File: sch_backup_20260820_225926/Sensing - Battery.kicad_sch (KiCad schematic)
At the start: 3 parts

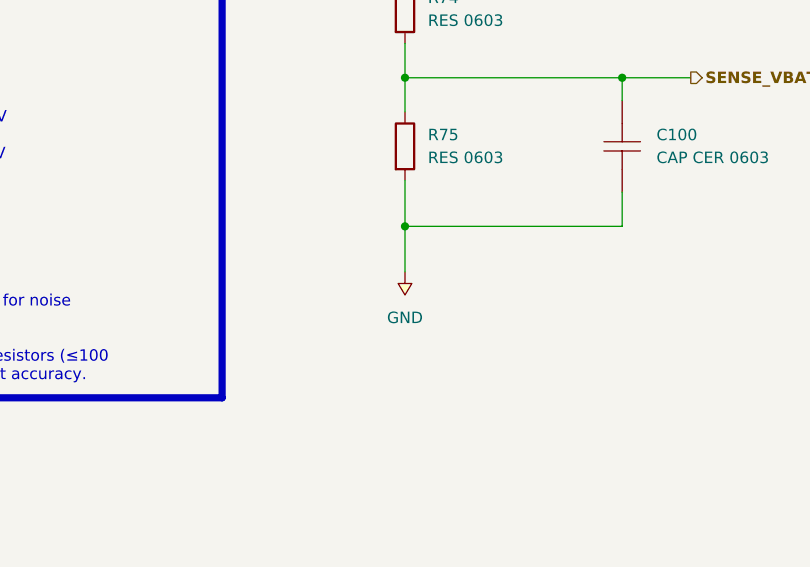
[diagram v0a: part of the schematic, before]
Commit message: Update Schematic
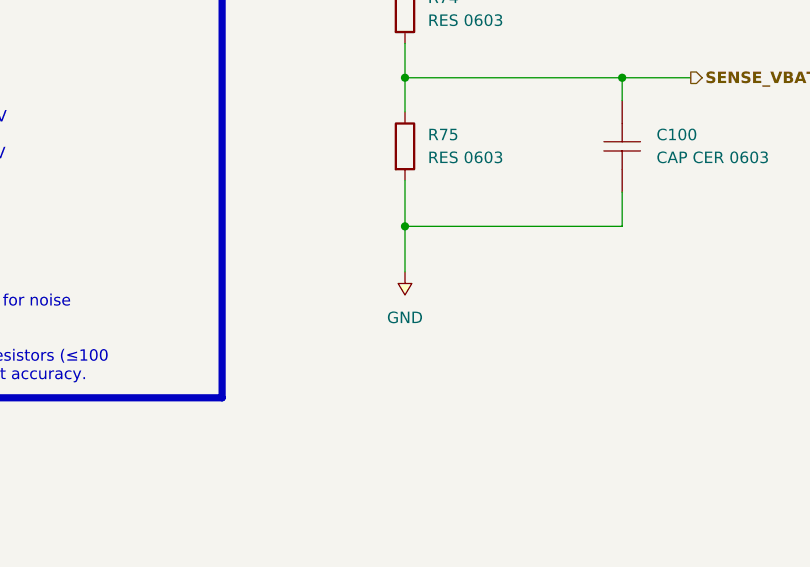
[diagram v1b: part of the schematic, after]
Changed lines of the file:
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@@
 	(symbol
 		(lib_id "Power_symbols:GND")
-		(at 168.91 102.87 0)
+		(at 166.37 101.6 180)
 		(unit 1)
 		(exclude_from_sim no)
@@
 		(dnp no)
 		(fields_autoplaced yes)
-		(property "Reference" "#PWR0135"
-			(at 168.656 94.234 0)
+		(property "Reference" "#PWR131"
+			(at 166.37 101.6 0)
 			(do_not_autoplace yes)
 			(effects
@@
 		)
 		(property "Footprint" ""
-			(at 168.91 102.87 0)
+			(at 166.37 101.6 0)
 			(effects
 				(font
@@
 		)
 		(property "Datasheet" ""
-			(at 168.91 102.87 0)
+			(at 166.37 101.6 0)
 			(effects
 				(font
@@
 		)
 		(property "Description" "Power Symbol - Global Ground"
-			(at 168.91 109.728 0)
+			(at 166.37 101.6 0)
 			(effects
 				(font
@@
 			(project "Master_Hand_Kicad"
 				(path "/f9e05184-c88b-4a88-ae9c-ab2bdb32be7c/c5103ceb-5325-4a84-a025-9638a412984e/d30056b5-4391-456e-bc80-2bde1ca0d521"
-					(reference "#PWR0135")
+					(reference "#PWR131")
 					(unit 1)
 				)
